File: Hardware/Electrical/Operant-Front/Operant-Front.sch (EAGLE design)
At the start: 16 parts, among them U1 CAT24C32

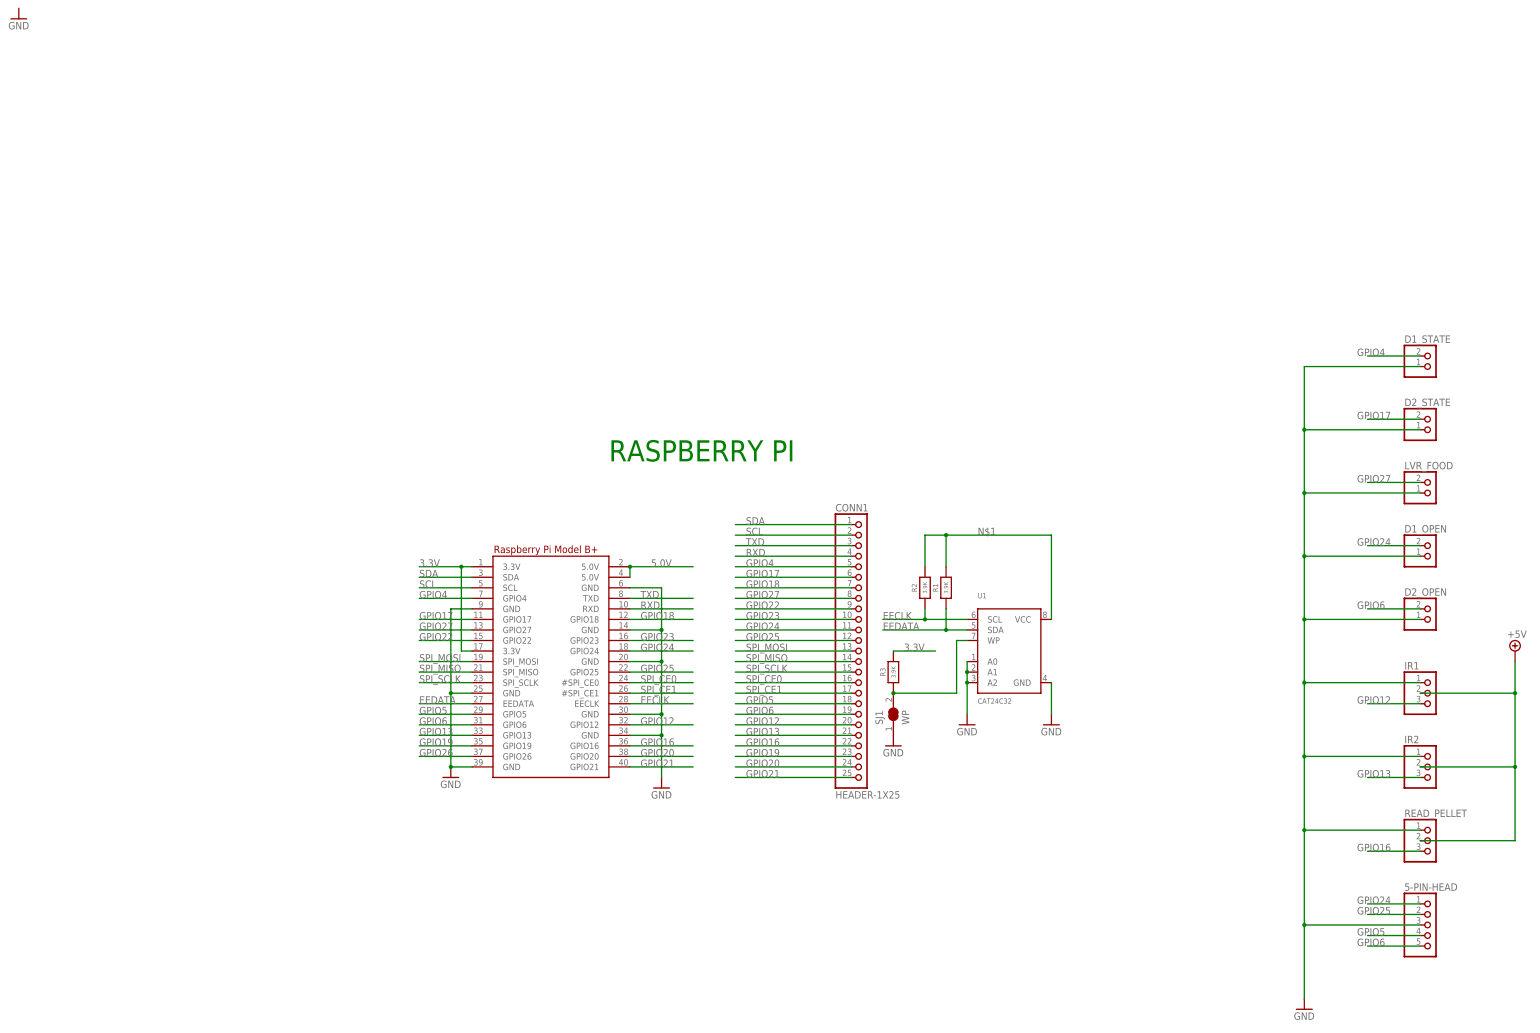
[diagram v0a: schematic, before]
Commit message: PCB Designs
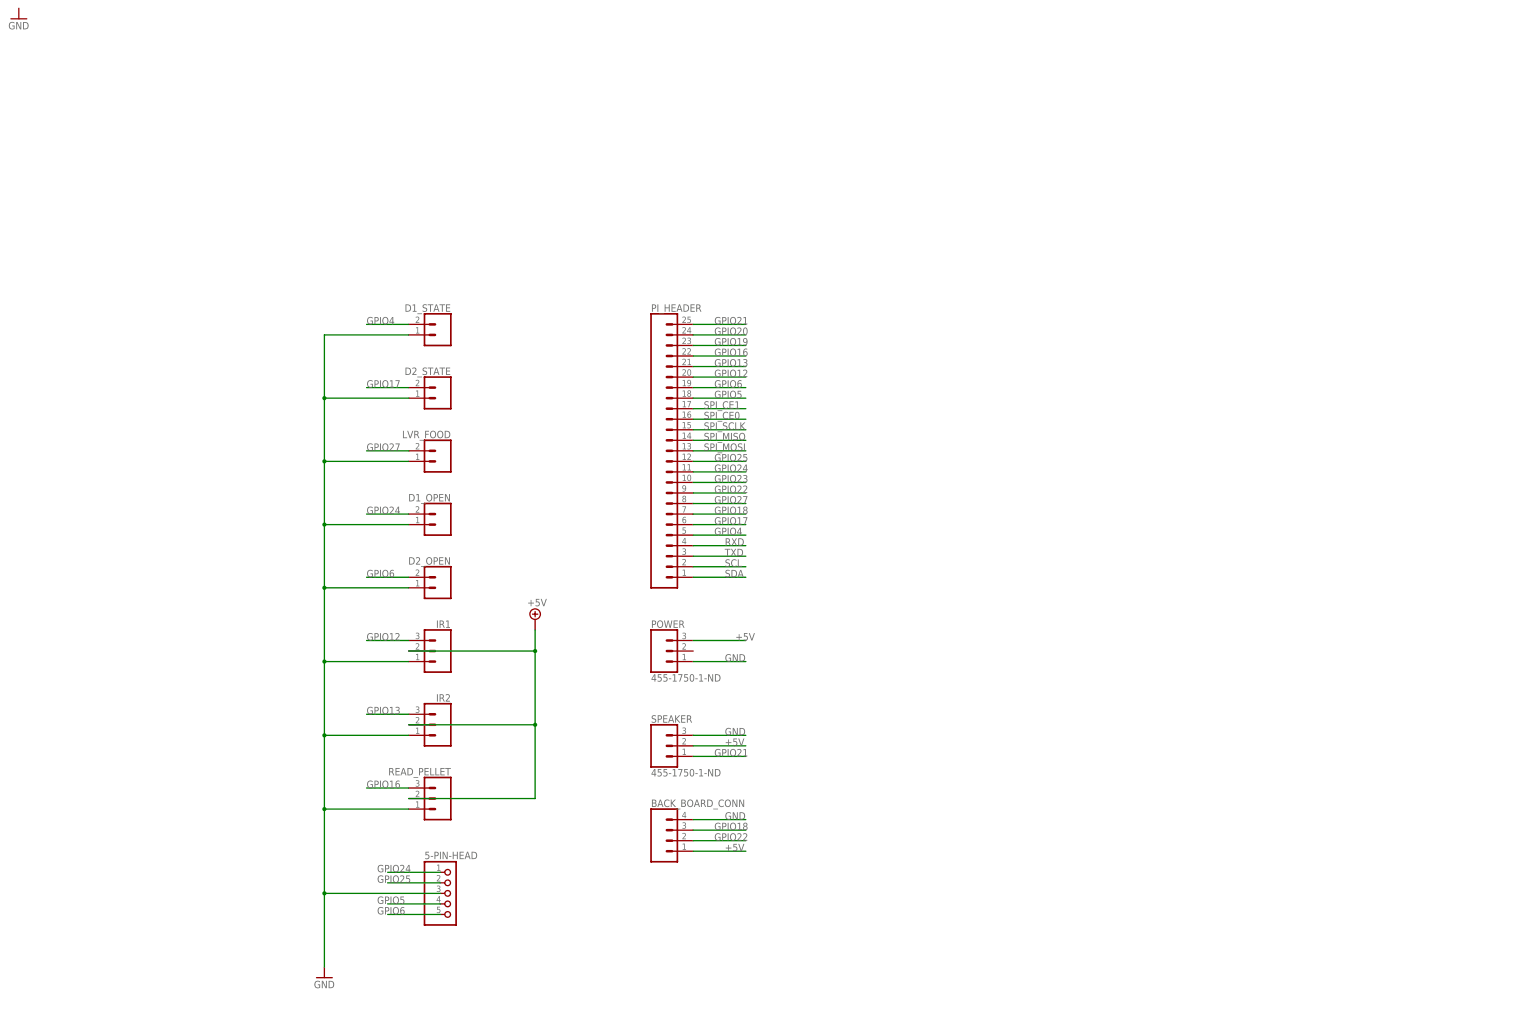
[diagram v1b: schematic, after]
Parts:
- removed CONN1: HEADER-1X25, microbuilder:HEADER-1X25
- removed R1, R2, R3: 3.9K, microbuilder:RESISTOR0805_NOOUTLINE
- removed RPI1: RASPBERRYPI_BPLUS_HATSLOTS, microbuilder:RASPBERRYPI_BPLUS_HATSLOTS
- removed SJ1: WP, microbuilder:SOLDERJUMPER_CLOSED
- removed U1: CAT24C32, microbuilder:EEPROM_I2C_SOIC8_GENERIC
- added BACK_BOARD_CONN: (no value), SparkFun-Connectors:CONN_04JST-PTH
- added PI_HEADER: (no value), SparkFun-Connectors:CONN_25
- added POWER, SPEAKER: 455-1750-1-ND, SparkFun-Connectors:CONN_03
- D1_OPEN, D1_STATE, D2_OPEN, D2_STATE, LVR_FOOD: device adafruit:JST_2PIN-SMT -> SparkFun-Connectors:CONN_02JST-PTH-2
- IR1, IR2, READ_PELLET: device adafruit:JST_3PIN -> SparkFun-Connectors:CONN_03JST-PTH
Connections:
- removed net 3.3V: R3.2, RPI1.3.3V, RPI1.3.3V@1
- removed net 5.0V: RPI1.5.0V, RPI1.5.0V@1
- removed net EECLK: R2.1, RPI1.EECLK, U1.SCL
- removed net EEDATA: R1.1, RPI1.EEDATA, U1.SDA
- removed net GPIO26: RPI1.GPIO26
- removed net N$1: R1.2, R2.2, U1.VCC
- removed net N$16: R3.1, SJ1.2, U1.WP
- net +5V: now also BACK_BOARD_CONN.1, POWER.3, SPEAKER.2
- net GND: now also BACK_BOARD_CONN.4, D1_OPEN.1, D1_STATE.1, D2_OPEN.1, D2_STATE.1, LVR_FOOD.1, POWER.1, SPEAKER.3; no longer D1_OPEN.2, D1_STATE.2, D2_OPEN.2, D2_STATE.2, LVR_FOOD.2, RPI1.GND, RPI1.GND@1, RPI1.GND@2, RPI1.GND@3, RPI1.GND@4, RPI1.GND@5, RPI1.GND@6, RPI1.GND@7, SJ1.1, U1.A0, U1.A1, U1.A2, U1.GND
- net GPIO12: now also PI_HEADER.20; no longer CONN1.20, RPI1.GPIO12
- net GPIO13: now also PI_HEADER.21; no longer CONN1.21, RPI1.GPIO13
- net GPIO16: now also PI_HEADER.22; no longer CONN1.22, RPI1.GPIO16
- net GPIO17: now also D2_STATE.2, PI_HEADER.6; no longer CONN1.6, D2_STATE.1, RPI1.GPIO17
- net GPIO18: now also BACK_BOARD_CONN.3, PI_HEADER.7; no longer CONN1.7, RPI1.GPIO18
- net GPIO19: now also PI_HEADER.23; no longer CONN1.23, RPI1.GPIO19
- net GPIO20: now also PI_HEADER.24; no longer CONN1.24, RPI1.GPIO20
- net GPIO21: now also PI_HEADER.25, SPEAKER.1; no longer CONN1.25, RPI1.GPIO21
- net GPIO22: now also BACK_BOARD_CONN.2, PI_HEADER.9; no longer CONN1.9, RPI1.GPIO22
- net GPIO23: now also PI_HEADER.10; no longer CONN1.10, RPI1.GPIO23
- net GPIO24: now also D1_OPEN.2, PI_HEADER.11; no longer CONN1.11, D1_OPEN.1, RPI1.GPIO24
- net GPIO25: now also PI_HEADER.12; no longer CONN1.12, RPI1.GPIO25
- net GPIO27: now also LVR_FOOD.2, PI_HEADER.8; no longer CONN1.8, LVR_FOOD.1, RPI1.GPIO27
- net GPIO4: now also D1_STATE.2, PI_HEADER.5; no longer CONN1.5, D1_STATE.1, RPI1.GPIO4
- net GPIO5: now also PI_HEADER.18; no longer CONN1.18, RPI1.GPIO5
- net GPIO6: now also D2_OPEN.2, PI_HEADER.19; no longer CONN1.19, D2_OPEN.1, RPI1.GPIO6
- net RXD: now also PI_HEADER.4; no longer CONN1.4, RPI1.RXD
- net SCL: now also PI_HEADER.2; no longer CONN1.2, RPI1.SCL
- net SDA: now also PI_HEADER.1; no longer CONN1.1, RPI1.SDA
- net SPI_CE0: now also PI_HEADER.16; no longer CONN1.16, RPI1.#SPI_CE0
- net SPI_CE1: now also PI_HEADER.17; no longer CONN1.17, RPI1.#SPI_CE1
- net SPI_MISO: now also PI_HEADER.14; no longer CONN1.14, RPI1.SPI_MISO
- net SPI_MOSI: now also PI_HEADER.13; no longer CONN1.13, RPI1.SPI_MOSI
- net SPI_SCLK: now also PI_HEADER.15; no longer CONN1.15, RPI1.SPI_SCLK
- net TXD: now also PI_HEADER.3; no longer CONN1.3, RPI1.TXD
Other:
- note removed: "RASPBERRY PI"
- moved on the sheet: 5-PIN-HEAD, D1_OPEN, D1_STATE, D2_OPEN, D2_STATE, LVR_FOOD
